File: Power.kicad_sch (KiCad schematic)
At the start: 36 parts, among them IC1 LMR33640DDDAR, J13 SM02B-GHS-TB, J16 SM02B-GHS-TB, J17 Screw_Terminal_01x02, Q1 SI2369BDS-T1-GE3 30V 5.6A, U3 AP7361C-33ER-13

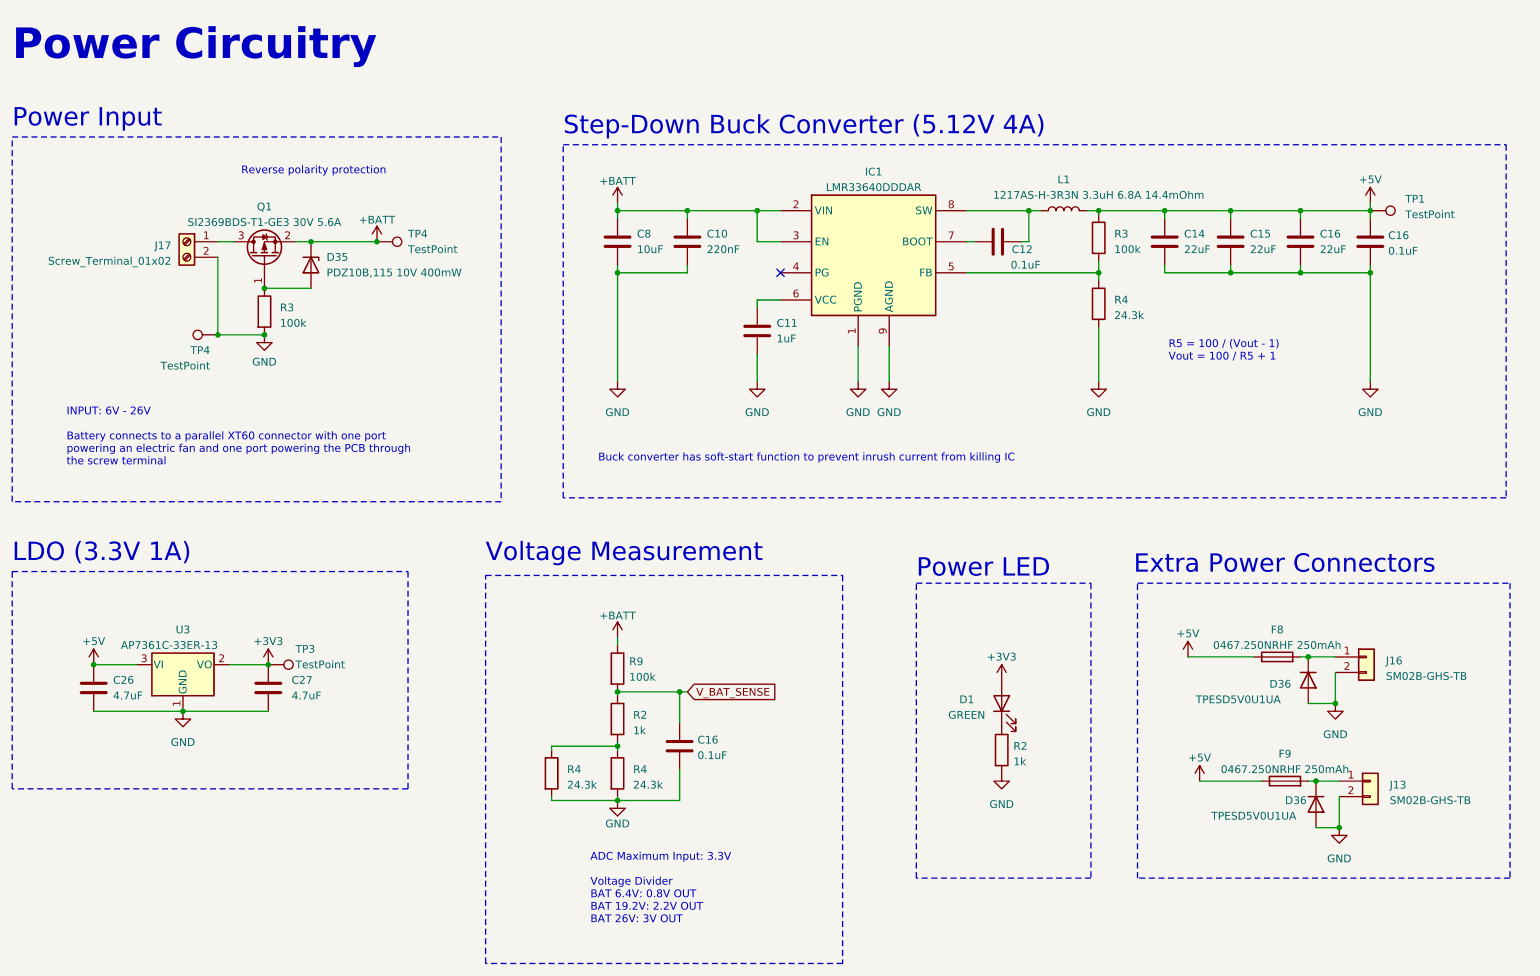
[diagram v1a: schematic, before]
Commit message: Add files via upload
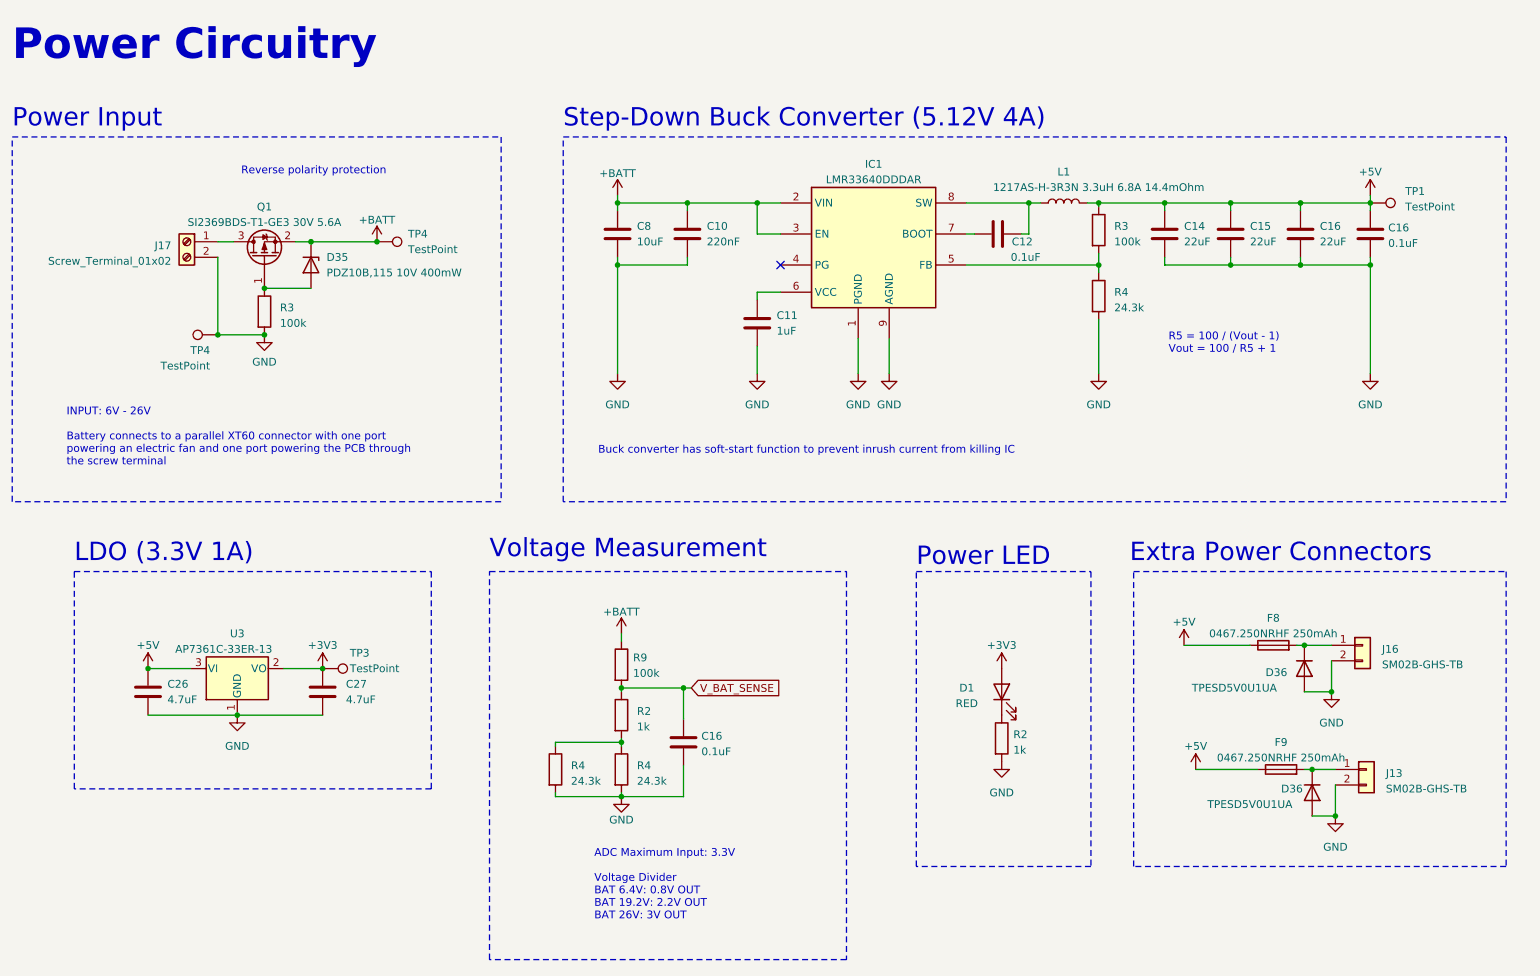
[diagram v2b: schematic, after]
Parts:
- D1: value GREEN -> RED
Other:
- moved on the sheet: C10, C11, C12, C14, C15, C16, C26, C27, C8, D1, D36, F8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
